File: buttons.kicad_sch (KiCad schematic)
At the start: 48 parts, among them SW10 SW_MEC_5G, SW11 SW_MEC_5G, SW12 SW_MEC_5G, SW13 SW_MEC_5G, SW14 SW_MEC_5G, SW15 SW_MEC_5G, SW16 SW_MEC_5G, SW17 SW_MEC_5G, SW18 SW_MEC_5G, SW19 SW_MEC_5G, SW2 SW_MEC_5G, SW20 SW_MEC_5G, SW21 SW_MEC_5G, SW22 SW_MEC_5G, SW23 SW_MEC_5G, SW24 SW_MEC_5G, SW25 SW_MEC_5G, SW3 SW_MEC_5G, SW4 SW_MEC_5G, SW5 SW_MEC_5G, SW6 SW_MEC_5G, SW7 SW_MEC_5G, SW8 SW_MEC_5G, SW9 SW_MEC_5G

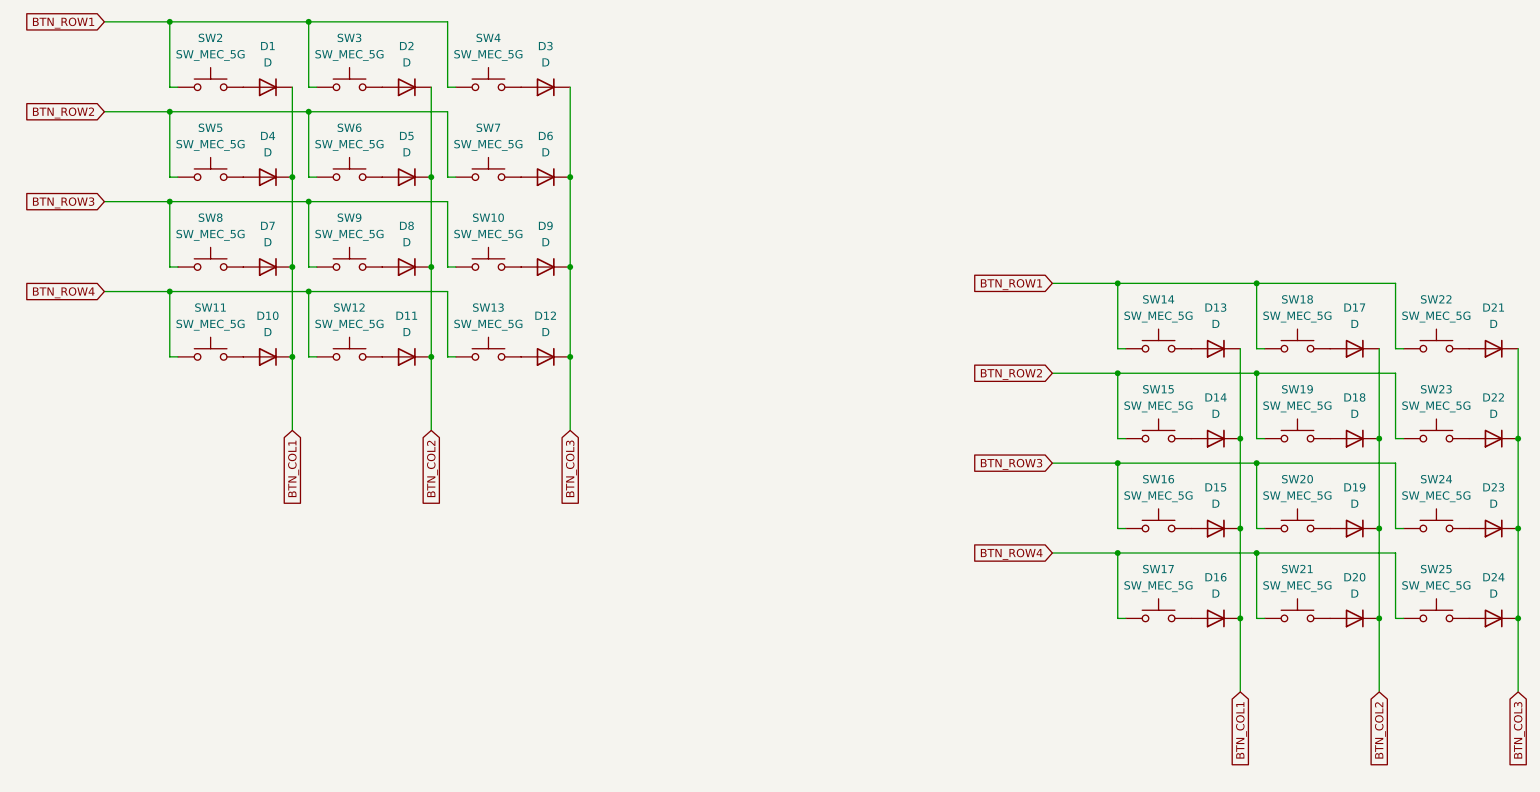
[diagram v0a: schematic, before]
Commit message: progress
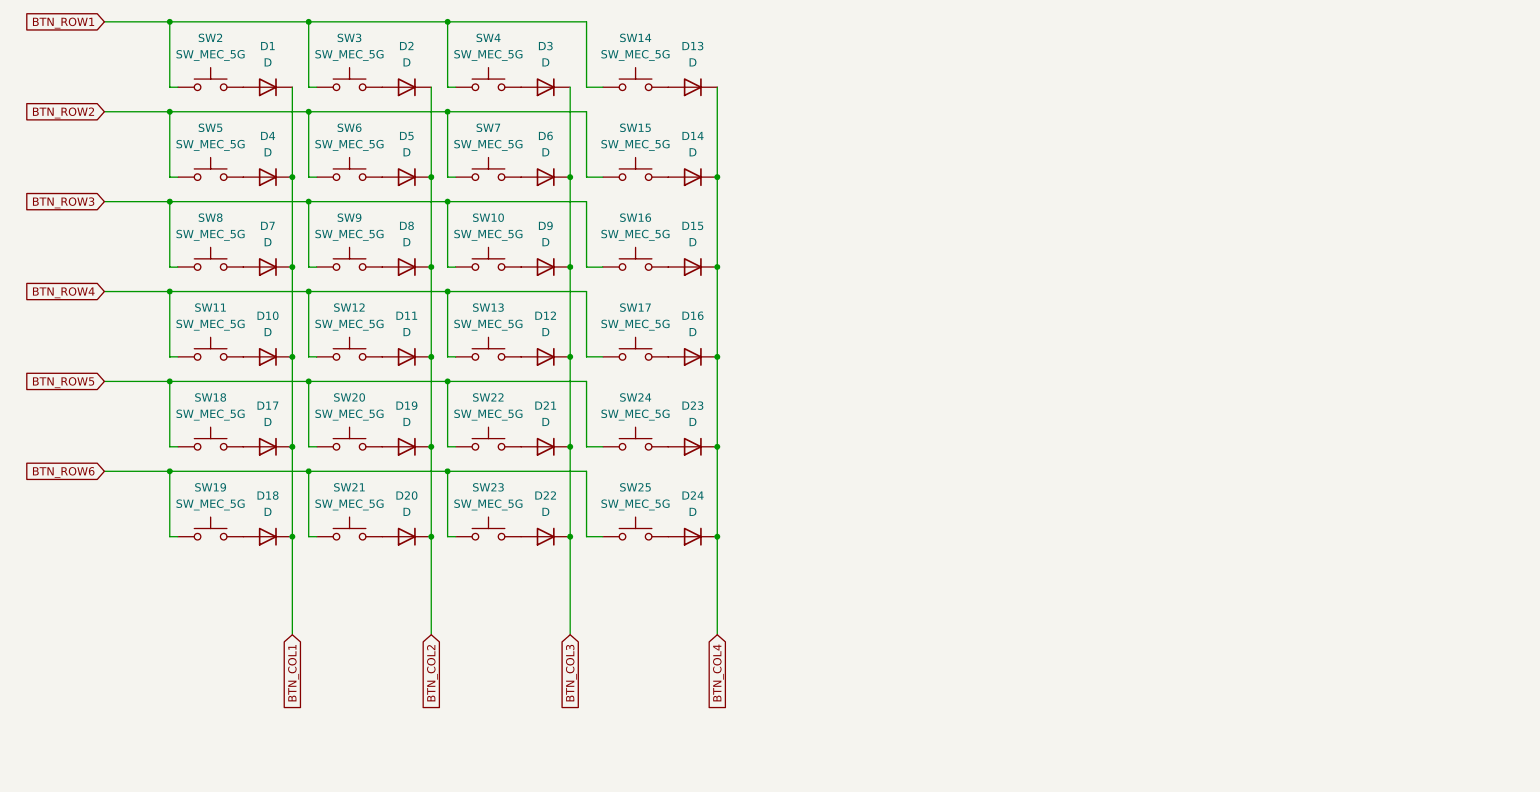
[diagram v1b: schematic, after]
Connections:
- net BTN_COL1: now also D17.1 (K), D18.1 (K); no longer D13.1 (K), D14.1 (K), D15.1 (K), D16.1 (K)
- net BTN_COL2: no longer D17.1 (K), D18.1 (K)
- net BTN_COL3: no longer D23.1 (K), D24.1 (K)
- net BTN_ROW1: no longer SW18.1 (A), SW18.2 (A), SW22.1 (A), SW22.2 (A)
- net BTN_ROW2: no longer SW19.1 (A), SW19.2 (A), SW23.1 (A), SW23.2 (A)
- net BTN_ROW3: no longer SW20.1 (A), SW20.2 (A), SW24.1 (A), SW24.2 (A)
- net BTN_ROW4: no longer SW21.1 (A), SW21.2 (A), SW25.1 (A), SW25.2 (A)
- new net BTN_COL4: D13.1 (K), D14.1 (K), D15.1 (K), D16.1 (K), D23.1 (K), D24.1 (K)
- new net BTN_ROW5: SW18.1 (A), SW18.2 (A), SW20.1 (A), SW20.2 (A), SW22.1 (A), SW22.2 (A), SW24.1 (A), SW24.2 (A)
- new net BTN_ROW6: SW19.1 (A), SW19.2 (A), SW21.1 (A), SW21.2 (A), SW23.1 (A), SW23.2 (A), SW25.1 (A), SW25.2 (A)

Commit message: progress
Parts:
- D1, D10, D11, D12, D13, D14, D15, D16, D17, D18, D19, D2, D20, D21, D22, D23, D24, D3, D4, D5, D6, D7, D8, D9: footprint (none) -> Diode_SMD:D_0201_0603Metric
- SW10, SW11, SW12, SW13, SW14, SW15, SW16, SW17, SW18, SW19, SW2, SW20, SW21, SW22, SW23, SW24, SW25, SW3, SW4, SW5, SW6, SW7, SW8, SW9: footprint (none) -> Button_Switch_SMD:SW_DIP_SPSTx01_Slide_6.7x4.1mm_W6.73mm_P2.54mm_LowProfile_JPin
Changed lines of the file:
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@@
 			)
 		)
-		(property "Footprint" ""
+		(property "Footprint" "Button_Switch_SMD:SW_DIP_SPSTx01_Slide_6.7x4.1mm_W6.73mm_P2.54mm_LowProfile_JPin"
 			(at 120.65 86.36 0)
 			(effects
@@
 			)
 		)
-		(property "Footprint" ""
+		(property "Footprint" "Button_Switch_SMD:SW_DIP_SPSTx01_Slide_6.7x4.1mm_W6.73mm_P2.54mm_LowProfile_JPin"
 			(at 54.61 100.33 0)
 			(effects
@@
 			)
 		)
-		(property "Footprint" ""
+		(property "Footprint" "Diode_SMD:D_0201_0603Metric"
 			(at 85.09 35.56 0)
 			(effects
@@
 			)
 		)
-		(property "Footprint" ""
+		(property "Footprint" "Diode_SMD:D_0201_0603Metric"
 			(at 106.68 63.5 0)
 			(effects
@@
 			)
 		)
-		(property "Footprint" ""
+		(property "Footprint" "Button_Switch_SMD:SW_DIP_SPSTx01_Slide_6.7x4.1mm_W6.73mm_P2.54mm_LowProfile_JPin"
 			(at 120.65 30.48 0)
 			(effects
@@
 			)
 		)
-		(property "Footprint" ""
+		(property "Footprint" "Diode_SMD:D_0201_0603Metric"
 			(at 106.68 35.56 0)
 			(effects
@@
 			)
 		)
-		(property "Footprint" ""
+		(property "Footprint" "Diode_SMD:D_0201_0603Metric"
 			(at 85.09 77.47 0)
 			(effects
@@
 			)
 		)
-		(property "Footprint" ""
+		(property "Footprint" "Button_Switch_SMD:SW_DIP_SPSTx01_Slide_6.7x4.1mm_W6.73mm_P2.54mm_LowProfile_JPin"
 			(at 97.79 100.33 0)
 			(effects
@@
 			)
 		)
-		(property "Footprint" ""
+		(property "Footprint" "Diode_SMD:D_0201_0603Metric"
 			(at 63.5 91.44 0)
 			(effects
@@
 			)
 		)
-		(property "Footprint" ""
+		(property "Footprint" "Button_Switch_SMD:SW_DIP_SPSTx01_Slide_6.7x4.1mm_W6.73mm_P2.54mm_LowProfile_JPin"
 			(at 76.2 72.39 0)
 			(effects
@@
 			)
 		)
-		(property "Footprint" ""
+		(property "Footprint" "Diode_SMD:D_0201_0603Metric"
 			(at 129.54 105.41 0)
 			(effects
@@
 			)
 		)
-		(property "Footprint" ""
+		(property "Footprint" "Diode_SMD:D_0201_0603Metric"
 			(at 85.09 63.5 0)
 			(effects
@@
 			)
 		)
-		(property "Footprint" ""
+		(property "Footprint" "Diode_SMD:D_0201_0603Metric"
 			(at 63.5 35.56 0)
 			(effects
@@
 			)
 		)
-		(property "Footprint" ""
+		(property "Footprint" "Diode_SMD:D_0201_0603Metric"
 			(at 63.5 105.41 0)
 			(effects
@@
 			)
 		)
-		(property "Footprint" ""
+		(property "Footprint" "Button_Switch_SMD:SW_DIP_SPSTx01_Slide_6.7x4.1mm_W6.73mm_P2.54mm_LowProfile_JPin"
 			(at 120.65 58.42 0)
 			(effects
@@
 			)
 		)
-		(property "Footprint" ""
+		(property "Footprint" "Diode_SMD:D_0201_0603Metric"
 			(at 129.54 49.53 0)
 			(effects
@@
 			)
 		)
-		(property "Footprint" ""
+		(property "Footprint" "Diode_SMD:D_0201_0603Metric"
 			(at 106.68 105.41 0)
 			(effects
@@
 			)
 		)
-		(property "Footprint" ""
+		(property "Footprint" "Button_Switch_SMD:SW_DIP_SPSTx01_Slide_6.7x4.1mm_W6.73mm_P2.54mm_LowProfile_JPin"
 			(at 76.2 30.48 0)
 			(effects
@@
 			)
 		)
-		(property "Footprint" ""
+		(property "Footprint" "Diode_SMD:D_0201_0603Metric"
 			(at 129.54 63.5 0)
 			(effects
@@
 			)
 		)
-		(property "Footprint" ""
+		(property "Footprint" "Button_Switch_SMD:SW_DIP_SPSTx01_Slide_6.7x4.1mm_W6.73mm_P2.54mm_LowProfile_JPin"
 			(at 76.2 44.45 0)
 			(effects
@@
 			)
 		)
-		(property "Footprint" ""
+		(property "Footprint" "Button_Switch_SMD:SW_DIP_SPSTx01_Slide_6.7x4.1mm_W6.73mm_P2.54mm_LowProfile_JPin"
 			(at 97.79 86.36 0)
 			(effects
@@
 			)
 		)
-		(property "Footprint" ""
+		(property "Footprint" "Button_Switch_SMD:SW_DIP_SPSTx01_Slide_6.7x4.1mm_W6.73mm_P2.54mm_LowProfile_JPin"
 			(at 76.2 58.42 0)
 			(effects
@@
 			)
 		)
-		(property "Footprint" ""
+		(property "Footprint" "Button_Switch_SMD:SW_DIP_SPSTx01_Slide_6.7x4.1mm_W6.73mm_P2.54mm_LowProfile_JPin"
 			(at 97.79 44.45 0)
 			(effects
@@
 			)
 		)
-		(property "Footprint" ""
+		(property "Footprint" "Diode_SMD:D_0201_0603Metric"
 			(at 129.54 77.47 0)
 			(effects
@@
 			)
 		)
-		(property "Footprint" ""
+		(property "Footprint" "Button_Switch_SMD:SW_DIP_SPSTx01_Slide_6.7x4.1mm_W6.73mm_P2.54mm_LowProfile_JPin"
 			(at 54.61 86.36 0)
 			(effects
@@
 			)
 		)
-		(property "Footprint" ""
+		(property "Footprint" "Button_Switch_SMD:SW_DIP_SPSTx01_Slide_6.7x4.1mm_W6.73mm_P2.54mm_LowProfile_JPin"
 			(at 76.2 86.36 0)
 			(effects
@@
 			)
 		)
-		(property "Footprint" ""
+		(property "Footprint" "Diode_SMD:D_0201_0603Metric"
 			(at 106.68 49.53 0)
 			(effects
@@
 			)
 		)
-		(property "Footprint" ""
+		(property "Footprint" "Button_Switch_SMD:SW_DIP_SPSTx01_Slide_6.7x4.1mm_W6.73mm_P2.54mm_LowProfile_JPin"
 			(at 76.2 100.33 0)
 			(effects
@@
 			)
 		)
-		(property "Footprint" ""
+		(property "Footprint" "Diode_SMD:D_0201_0603Metric"
 			(at 129.54 91.44 0)
 			(effects
@@
 			)
 		)
-		(property "Footprint" ""
+		(property "Footprint" "Diode_SMD:D_0201_0603Metric"
 			(at 85.09 49.53 0)
 			(effects
@@
 			)
 		)
-		(property "Footprint" ""
+		(property "Footprint" "Diode_SMD:D_0201_0603Metric"
 			(at 63.5 49.53 0)
 			(effects
@@
 			)
 		)
-		(property "Footprint" ""
+		(property "Footprint" "Diode_SMD:D_0201_0603Metric"
 			(at 63.5 63.5 0)
 			(effects
@@
 			)
 		)
-		(property "Footprint" ""
+		(property "Footprint" "Diode_SMD:D_0201_0603Metric"
 			(at 63.5 77.47 0)
 			(effects
@@
 			)
 		)
-		(property "Footprint" ""
+		(property "Footprint" "Button_Switch_SMD:SW_DIP_SPSTx01_Slide_6.7x4.1mm_W6.73mm_P2.54mm_LowProfile_JPin"
 			(at 97.79 30.48 0)
 			(effects
@@
 			)
 		)
-		(property "Footprint" ""
+		(property "Footprint" "Button_Switch_SMD:SW_DIP_SPSTx01_Slide_6.7x4.1mm_W6.73mm_P2.54mm_LowProfile_JPin"
 			(at 97.79 58.42 0)
 			(effects
@@
 			)
 		)
-		(property "Footprint" ""
+		(property "Footprint" "Diode_SMD:D_0201_0603Metric"
 			(at 106.68 91.44 0)
 			(effects
@@
 			)
 		)
-		(property "Footprint" ""
+		(property "Footprint" "Button_Switch_SMD:SW_DIP_SPSTx01_Slide_6.7x4.1mm_W6.73mm_P2.54mm_LowProfile_JPin"
 			(at 54.61 72.39 0)
 			(effects
@@
 			)
 		)
-		(property "Footprint" ""
+		(property "Footprint" "Button_Switch_SMD:SW_DIP_SPSTx01_Slide_6.7x4.1mm_W6.73mm_P2.54mm_LowProfile_JPin"
 			(at 120.65 72.39 0)
 			(effects
@@
 			)
 		)
-		(property "Footprint" ""
+		(property "Footprint" "Button_Switch_SMD:SW_DIP_SPSTx01_Slide_6.7x4.1mm_W6.73mm_P2.54mm_LowProfile_JPin"
 			(at 54.61 30.48 0)
 			(effects
@@
 			)
 		)
-		(property "Footprint" ""
+		(property "Footprint" "Button_Switch_SMD:SW_DIP_SPSTx01_Slide_6.7x4.1mm_W6.73mm_P2.54mm_LowProfile_JPin"
 			(at 120.65 100.33 0)
 			(effects
@@
 			)
 		)
-		(property "Footprint" ""
+		(property "Footprint" "Diode_SMD:D_0201_0603Metric"
 			(at 85.09 105.41 0)
 			(effects
@@
 			)
 		)
-		(property "Footprint" ""
+		(property "Footprint" "Button_Switch_SMD:SW_DIP_SPSTx01_Slide_6.7x4.1mm_W6.73mm_P2.54mm_LowProfile_JPin"
 			(at 54.61 58.42 0)
 			(effects
@@
 			)
 		)
-		(property "Footprint" ""
+		(property "Footprint" "Button_Switch_SMD:SW_DIP_SPSTx01_Slide_6.7x4.1mm_W6.73mm_P2.54mm_LowProfile_JPin"
 			(at 120.65 44.45 0)
 			(effects
@@
 			)
 		)
-		(property "Footprint" ""
+		(property "Footprint" "Button_Switch_SMD:SW_DIP_SPSTx01_Slide_6.7x4.1mm_W6.73mm_P2.54mm_LowProfile_JPin"
 			(at 97.79 72.39 0)
 			(effects
@@
 			)
 		)
-		(property "Footprint" ""
+		(property "Footprint" "Diode_SMD:D_0201_0603Metric"
 			(at 85.09 91.44 0)
 			(effects
@@
 			)
 		)
-		(property "Footprint" ""
+		(property "Footprint" "Button_Switch_SMD:SW_DIP_SPSTx01_Slide_6.7x4.1mm_W6.73mm_P2.54mm_LowProfile_JPin"
 			(at 54.61 44.45 0)
 			(effects
@@
 			)
 		)
-		(property "Footprint" ""
+		(property "Footprint" "Diode_SMD:D_0201_0603Metric"
 			(at 106.68 77.47 0)
 			(effects
@@
 			)
 		)
-		(property "Footprint" ""
+		(property "Footprint" "Diode_SMD:D_0201_0603Metric"
 			(at 129.54 35.56 0)
 			(effects
